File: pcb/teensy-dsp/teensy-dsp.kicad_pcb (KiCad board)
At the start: 4 copper layers, 101 x 82 mm, 14 parts, among them J1 ACJS-IH, J2 ACJS-IH, J3 FSW1, J4 FSW2, J5 ACJS-IH, J6 ACJS-IH, J7 Conn_02x15_Odd_Even, J8 Barrel_Jack_Switch, J9 USB_B_Mini, U1 Teensy4.1, U2 Teensy4.0_AudioShield_REVD, U3 LM7805_TO220

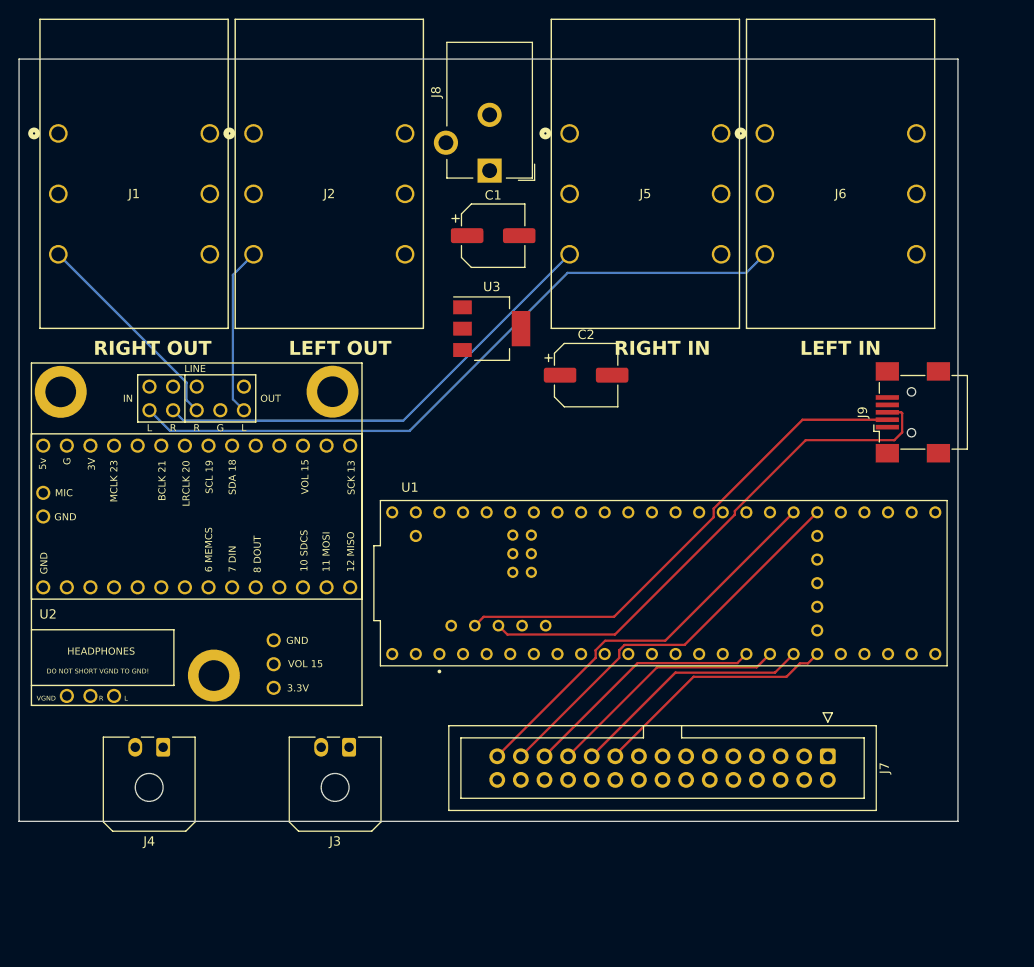
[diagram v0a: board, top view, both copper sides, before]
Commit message: update pcb layout
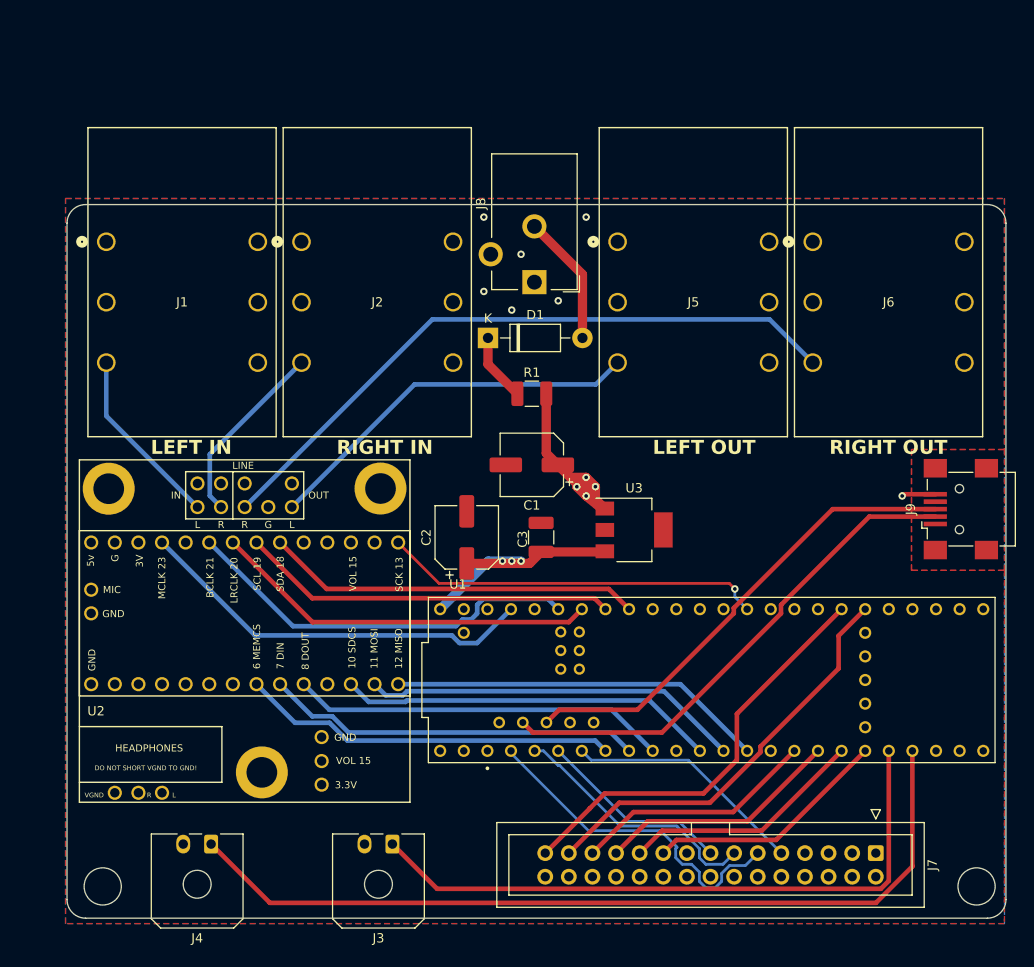
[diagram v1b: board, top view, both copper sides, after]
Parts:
- added C3: 100n 16V, Capacitor_SMD:C_1210_3225Metric_Pad1.33x2.70mm_HandSolder, F.Cu at (152.2, 100.5)
- added D1: D, Diode_THT:D_DO-41_SOD81_P10.16mm_Horizontal, F.Cu at (146.4, 79.0)
- added R1: 47R, Resistor_SMD:R_1210_3225Metric_Pad1.30x2.65mm_HandSolder, F.Cu at (151.2, 85.0)
- moved U3 26.5 mm to (162.2, 99.7)
- moved C1 25.0 mm to (151.2, 92.7), turned to 180 degrees
- moved C2 21.7 mm to (144.2, 100.5), turned to 90 degrees
- moved J8 12.9 mm to (151.4, 73.0)
- moved J1 12.7 mm to (105.4, 68.7)
- moved J2 12.7 mm to (126.4, 68.7)
- moved J5 12.7 mm to (160.4, 68.7)
- moved J6 12.7 mm to (181.4, 68.7)
- moved U2 11.6 mm to (103.8, 116.2)
- moved J9 11.6 mm to (197.2, 97.4)
- moved U1 11.6 mm to (170.5, 115.8)
- moved J4 11.6 mm to (116.7, 133.4)
- moved J7 11.6 mm to (188.2, 134.4)
- moved J3 11.4 mm to (136.2, 133.4)
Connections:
- J1 pad T: R Line Out -> L Line In
- J2 pad T: L Line Out -> R Line In
- J5 pad T: R Line In -> L Line Out
- J6 pad T: L Line In -> R Line Out
- J8 pad 2: +9V -> Net-(D1-A)
- J9 pad 6: unconnected-(J9-Shield-Pad6) -> Earth
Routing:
- net +5V: track 0.00 -> 127.2 mm, vias 0 -> 3
- net +9V: track 0.00 -> 117.9 mm, vias 0 -> 4
- net FSW_2: track 0.00 -> 92.1 mm
- net FSW_1: track 0.00 -> 69.7 mm
- net L Line In: track 75.0 -> 19.6 mm
- net R Line Out: track 22.9 -> 71.4 mm
- net Audio MCLK: track 0.00 -> 43.5 mm
- net Audio BCLK: track 0.00 -> 43.5 mm
- net Audio LRCLK: track 0.00 -> 41.7 mm
- net Audio SCK: track 0.00 -> 41.0 mm, vias 0 -> 1
- net Audio MOSI: track 0.00 -> 40.9 mm
- net Audio SDCS: track 0.00 -> 40.6 mm
- net Audio MEMCS: track 0.00 -> 40.5 mm
- net Audio SCL: track 0.00 -> 40.5 mm
- net Audio DOUT: track 0.00 -> 40.5 mm
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- added copper zone on F.Cu, net Earth
- added copper zone on B.Cu, net GND
- added copper zone on F.Cu, net GND
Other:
- board size 101 x 82 mm -> 101 x 76.8 mm
